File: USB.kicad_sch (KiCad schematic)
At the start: 26 parts, among them J11 USB3_A, U16 USB5744_2G, Y5 25Mhz

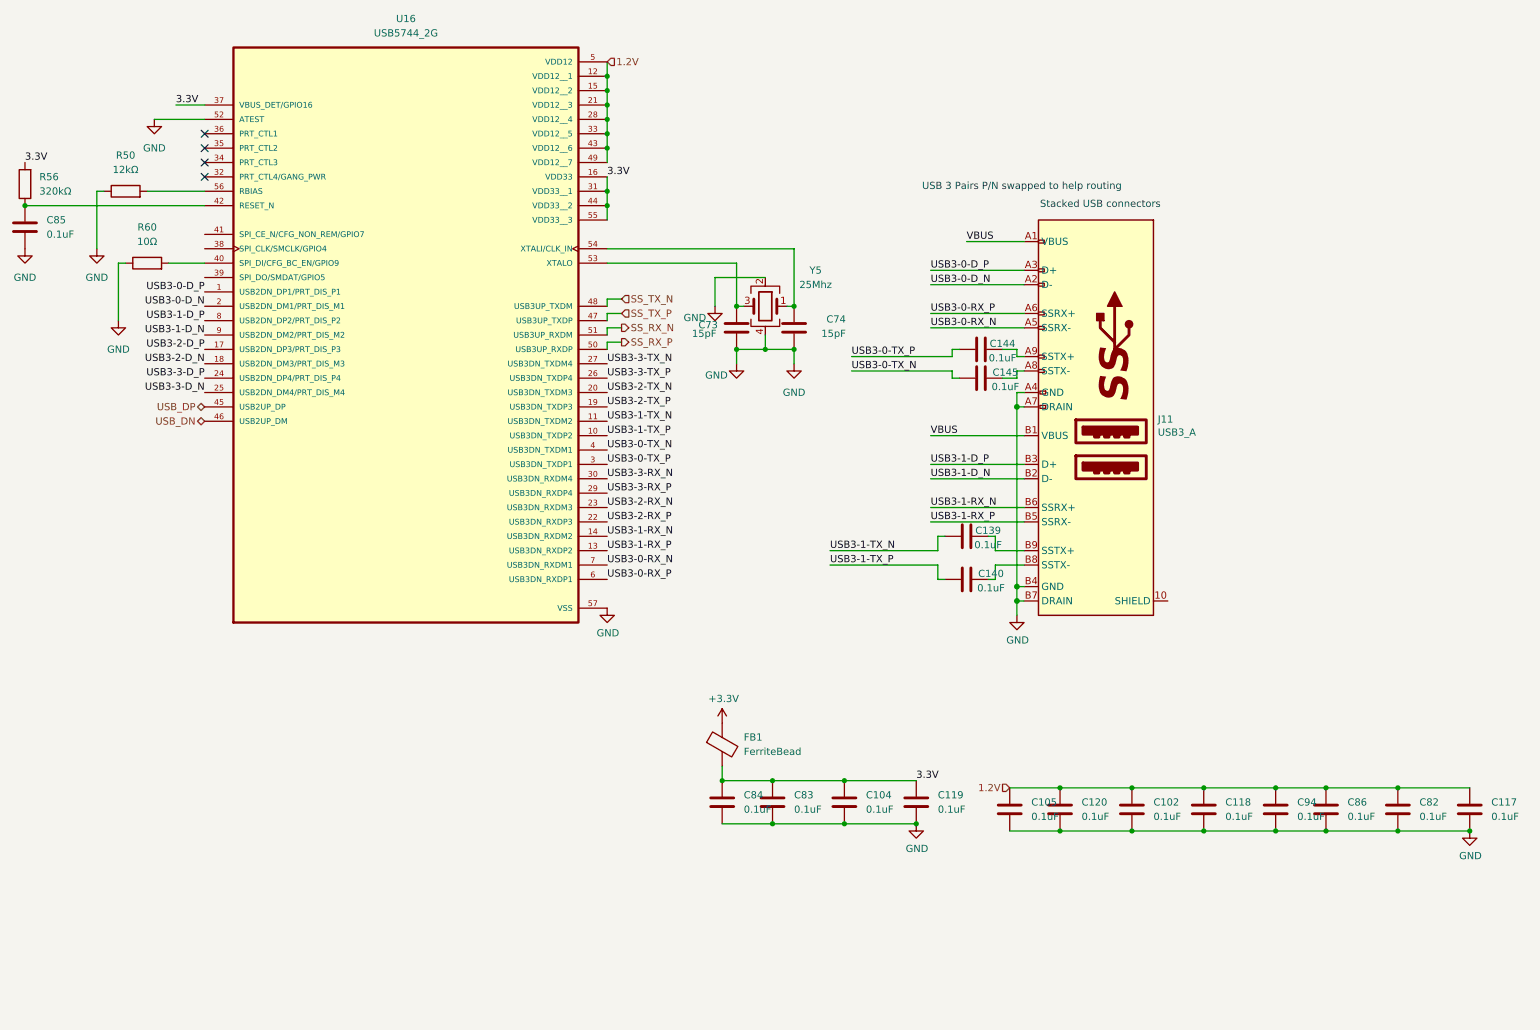
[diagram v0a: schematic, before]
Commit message: データをアップロード
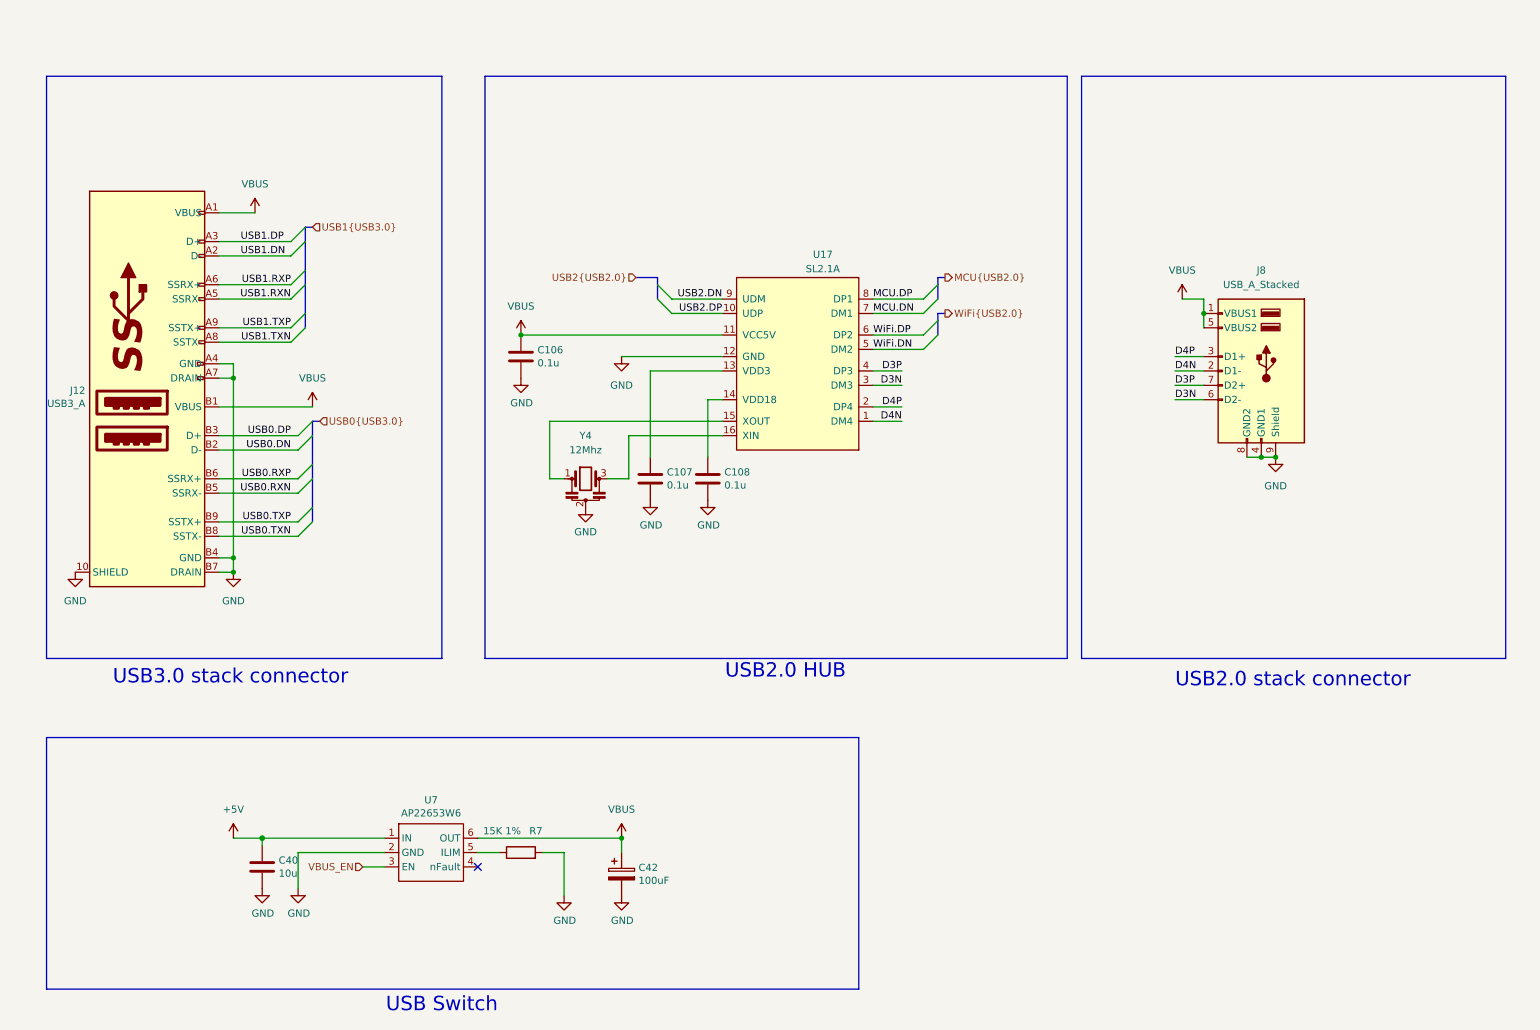
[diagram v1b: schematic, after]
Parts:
- removed C102, C104, C105, C117, C118, C119, C120, C139, C140, C144, C145, C82, C83, C84, C85, C86, C94: 0.1uF, Capacitor_SMD:C_0402_1005Metric_Pad0.74x0.62mm_HandSolder, symbol Device:C
- removed C73, C74: 15pF, Capacitor_SMD:C_0603_1608Metric_Pad1.08x0.95mm_HandSolder, symbol Device:C
- removed FB1: FerriteBead, Inductor_SMD:L_0603_1608Metric_Pad1.05x0.95mm_HandSolder, symbol Device:FerriteBead
- removed J11: USB3_A, CM5IO:MTCONN_UBAF30-D2011, symbol CM5IO:USB3_A
- removed R50: 12kΩ, Resistor_SMD:R_0603_1608Metric_Pad0.98x0.95mm_HandSolder, symbol Device:R
- removed R56: 320kΩ, Resistor_SMD:R_0603_1608Metric, symbol Device:R
- removed R60: 10Ω, Resistor_SMD:R_0603_1608Metric, symbol Device:R
- removed U16: USB5744_2G, CM5IO:VQFN56_2G_MCH, symbol USB5744:USB5744_2G
- removed Y5: 25Mhz, Crystal:Crystal_SMD_SeikoEpson_FA128-4Pin_2.0x1.6mm, symbol Device:Crystal_GND24
- added C106, C107, C108: 0.1u, Capacitor_SMD:C_0402_1005Metric_Pad0.74x0.62mm_HandSolder, symbol Device:C
- added C40: 10u, Capacitor_SMD:C_0805_2012Metric, symbol Device:C
- added C42: 100uF, Capacitor_Tantalum_SMD:CP_EIA-7343-31_Kemet-D, symbol Device:C_Polarized
- added J12: USB3_A, CM5IO:MTCONN_UBAF30-D2011, symbol CM5IO:USB3_A
- added J8: USB_A_Stacked, Connector_USB:USB_A_Wuerth_61400826021_Horizontal_Stacked, symbol Connector:USB_A_Stacked
- added R7: 15K 1%, Resistor_SMD:R_0603_1608Metric_Pad0.98x0.95mm_HandSolder, symbol Device:R
- added U17: SL2.1A, Package_SO:SOIC-16_4.55x10.3mm_P1.27mm, symbol SL2.1A:SL2.1A
- added U7: AP22653W6, Package_TO_SOT_SMD:SOT-23-6, symbol CM5IO:AP2553W6
- added Y4: 12Mhz, Crystal:Resonator_SMD_Murata_CSTxExxV-3Pin_3.0x1.1mm, symbol Device:Resonator
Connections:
- net GND: now also C106.2, C107.2, C108.2, C40.2, C42.2, J12.10 (SHIELD), J12.A4 (GND), J12.A7 (DRAIN), J12.B4 (GND), J12.B7 (DRAIN), J8.4 (GND1), J8.8 (GND2), J8.9 (Shield), R7.2, U17.12 (GND), U7.2 (GND), Y4.2
- net VBUS: now also C106.1, C42.1, J12.A1 (VBUS), J12.B1 (VBUS), J8.1 (VBUS1), J8.5 (VBUS2), U17.11 (VCC5V), U7.6 (OUT)
- new net: U17.15 (XOUT), Y4.1
- new net: U17.16 (XIN), Y4.3
- new net: C108.1, U17.14 (VDD18)
- new net: C107.1, U17.13 (VDD3)
- new net: R7.1, U7.5 (ILIM)
- new net +5V: C40.1, U7.1 (IN)
- new net D3N: J8.6 (D2-), U17.3 (DM3)
- new net D3P: J8.7 (D2+), U17.4 (DP3)
- new net D4N: J8.2 (D1-), U17.1 (DM4)
- new net D4P: J8.3 (D1+), U17.2 (DP4)
- new net MCU.DN: U17.7 (DM1)
- new net MCU.DP: U17.8 (DP1)
- new net USB0.DN: J12.B2 (D-)
- new net USB0.DP: J12.B3 (D+)
- new net USB0.RXN: J12.B5 (SSRX-)
- new net USB0.RXP: J12.B6 (SSRX+)
- new net USB0.TXN: J12.B8 (SSTX-)
- new net USB0.TXP: J12.B9 (SSTX+)
- new net USB1.DN: J12.A2 (D-)
- new net USB1.DP: J12.A3 (D+)
- new net USB1.RXN: J12.A5 (SSRX-)
- new net USB1.RXP: J12.A6 (SSRX+)
- new net USB1.TXN: J12.A8 (SSTX-)
- new net USB1.TXP: J12.A9 (SSTX+)
- new net USB2.DN: U17.9 (UDM)
- new net USB2.DP: U17.10 (UDP)
- new net VBUS_EN: U7.3 (EN)
- new net WiFi.DN: U17.5 (DM2)
- new net WiFi.DP: U17.6 (DP2)
- no-connect marks 4 -> 1
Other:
- note added: "USB Switch"
- note added: "USB2.0 HUB"
- note added: "USB2.0 stack connector"
- note added: "USB3.0 stack connector"
- note removed: "Stacked USB connectors"
- note removed: "USB 3 Pairs P/N swapped to help routing"
